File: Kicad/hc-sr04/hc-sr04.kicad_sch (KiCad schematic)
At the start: 11 parts, among them IC1 MCP1755, K1 HC-SR04, K2 MCU

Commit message: Update HC-SR04
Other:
- title: TBOT - Front HC-SR04 -> TBOT - HC-SR04
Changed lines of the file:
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@@
   (paper "A4")
   (title_block
-    (title "TBOT - Front HC-SR04")
+    (title "TBOT - HC-SR04")
     (date "01/2022")
     (rev "A")

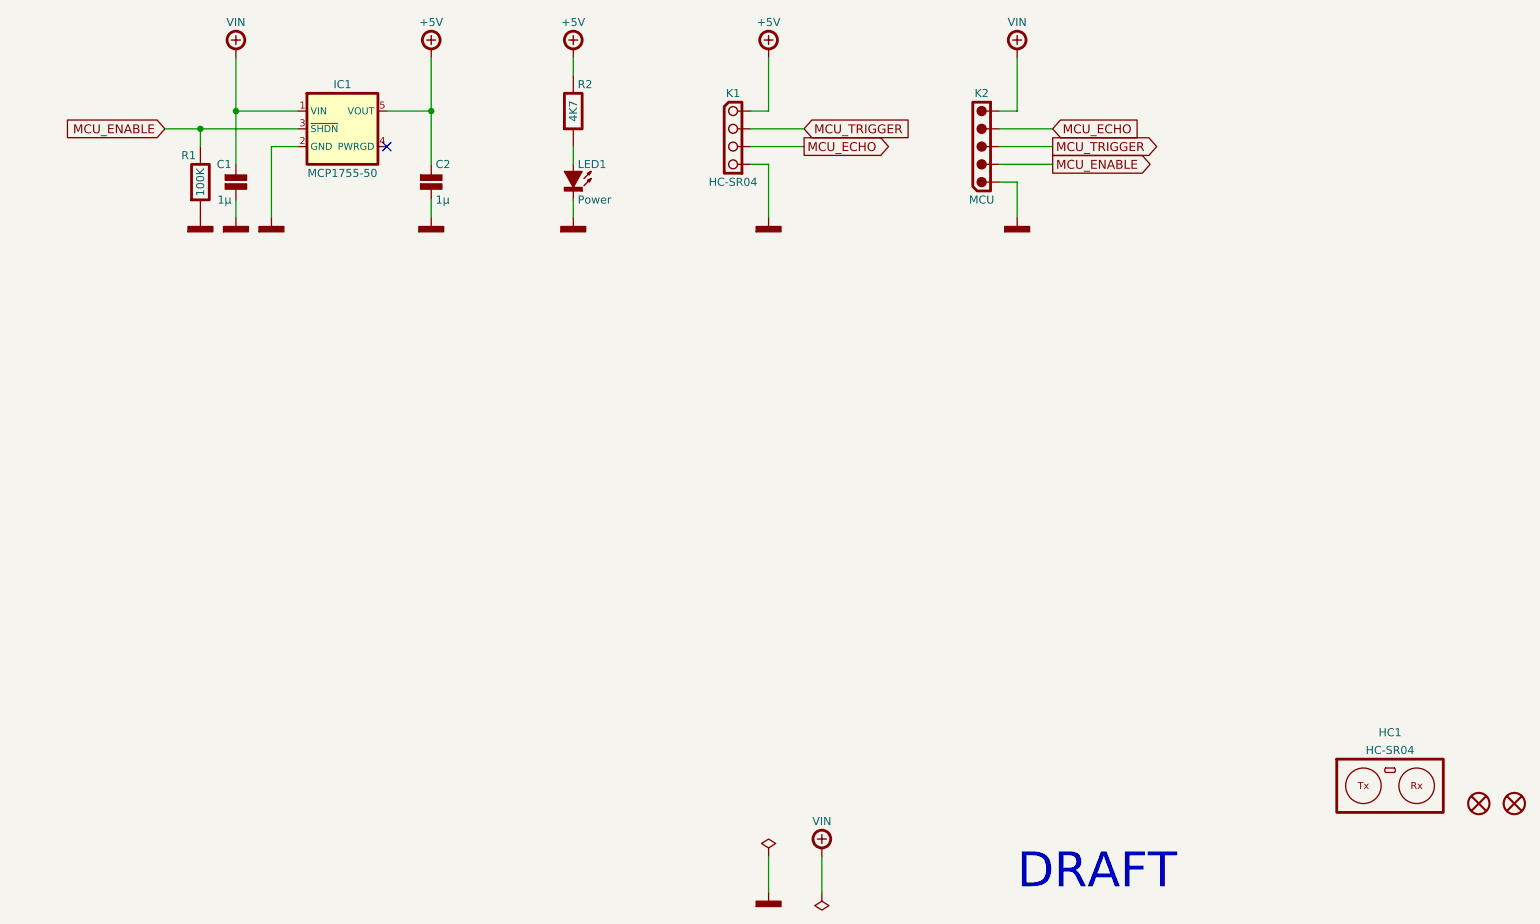
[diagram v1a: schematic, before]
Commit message: Update
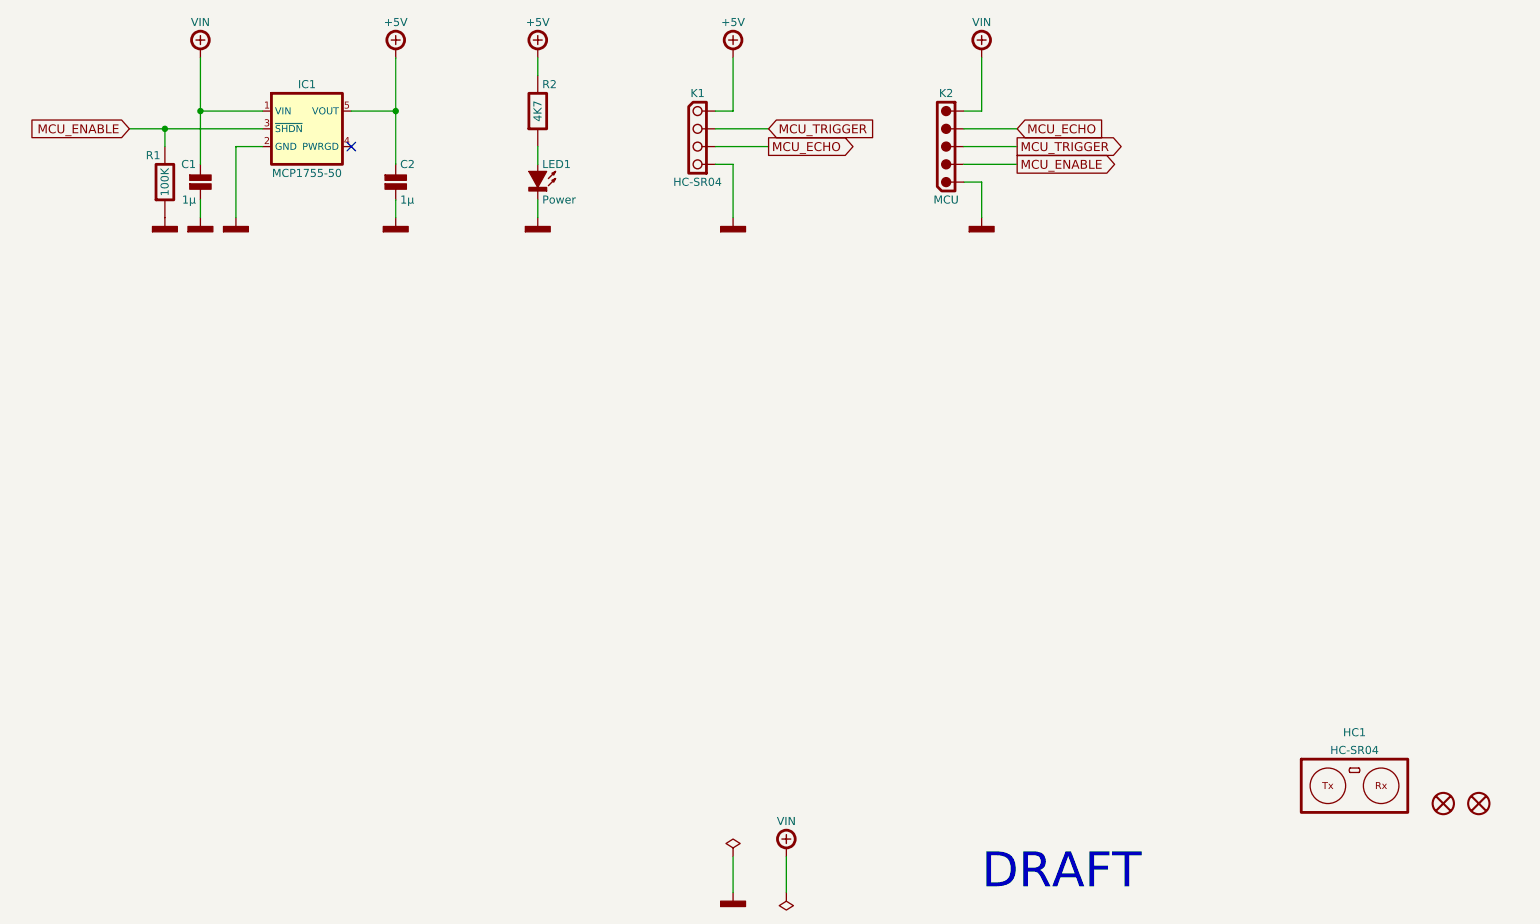
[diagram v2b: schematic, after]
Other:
- moved on the sheet: C1, C2, HC1, IC1, K1, K2, LED1, R1, R2
